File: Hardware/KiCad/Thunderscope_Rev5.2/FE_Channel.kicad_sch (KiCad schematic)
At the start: 103 parts, among them J1002_4 BNC, J3_4 UFL, J4_4 UFL, K1000_4 UD2-4.5NUN-L, K1001_4 UD2-4.5NUN-L, Q1002_4 DMN62D0UW, Q1003_4 DMN62D0UW, U1001_4 TMUX4053, U1008_4 LMH6518, U1009_4 BUF802, U1011_4 OPA140AIDBVR

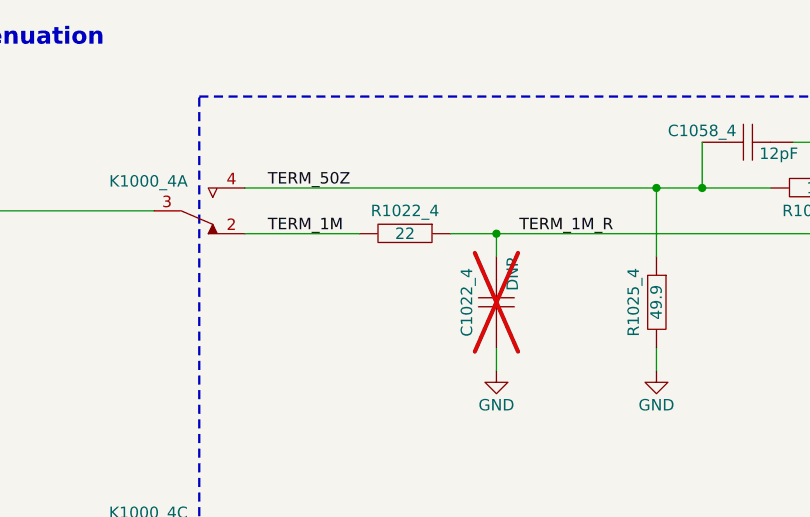
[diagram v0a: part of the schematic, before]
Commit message: Changed R1022 for #387
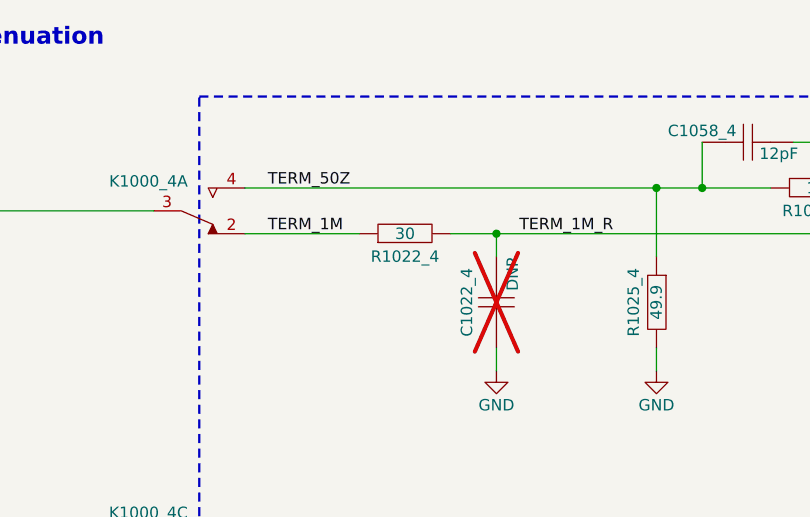
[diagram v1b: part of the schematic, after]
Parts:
- R1022_4: value 22 -> 30; symbol Thunderscope_Rev5:RES 22 OHM 1% 1/3W 0603 -> Thunderscope_Rev5:RES 30 OHM 1% 1/3W 0603; MANUFACTURER PART NUMBER SG73P1JTTD22R0F -> SG73P1JTTD30R0F; SUPPLIER PART NUMBER 1 660-SG73P1JTTD22R0F -> 660-SG73P1JTTD30R0F
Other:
- moved on the sheet: R1022_4
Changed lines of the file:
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@@
 	)
 	(symbol
-		(lib_id "Thunderscope_Rev5:RES 22 OHM 1% 1/3W 0603")
-		(at 91.44 38.1 0)
+		(lib_id "Thunderscope_Rev5:RES 30 OHM 1% 1/3W 0603")
+		(at 91.44 38.1 180)
 		(unit 1)
 		(exclude_from_sim no)
@@
 		(dnp no)
 		(property "Reference" "R1022_4"
-			(at 91.44 35.56 0)
+			(at 91.44 40.64 0)
 			(effects
 				(font
@@
 			)
 		)
-		(property "Value" "22"
+		(property "Value" "30"
 			(at 91.44 38.1 0)
 			(effects
@@
 		)
 		(property "TOLERANCE" "1%"
-			(at 88.392 46.736 0)
+			(at 94.488 29.464 0)
 			(effects
 				(font
@@
 		)
 		(property "PACKAGE" "0603"
-			(at 88.9 40.64 0)
+			(at 93.98 35.56 0)
 			(effects
 				(font
@@
 		)
 		(property "SUPPLIER 1" "Mouser"
-			(at 85.852 34.584 0)
+			(at 97.028 41.616 0)
 			(effects
 				(font
@@
 			)
 		)
-		(property "SUPPLIER PART NUMBER 1" "660-SG73P1JTTD22R0F"
-			(at 85.852 34.584 0)
+		(property "SUPPLIER PART NUMBER 1" "660-SG73P1JTTD30R0F"
+			(at 97.028 41.616 0)
 			(effects
 				(font
@@
 		)
 		(property "MANUFACTURER" "KOA Speer"
-			(at 85.852 34.584 0)
+			(at 97.028 41.616 0)
 			(effects
 				(font
@@
 		)
 		(property "HOUSE PART NUMBER" ""
-			(at 85.852 34.584 0)
+			(at 97.028 41.616 0)
 			(effects
 				(font
@@
 			)
 		)
-		(property "MANUFACTURER PART NUMBER" "SG73P1JTTD22R0F"
-			(at 85.852 34.584 0)
+		(property "MANUFACTURER PART NUMBER" "SG73P1JTTD30R0F"
+			(at 97.028 41.616 0)
 			(effects
 				(font

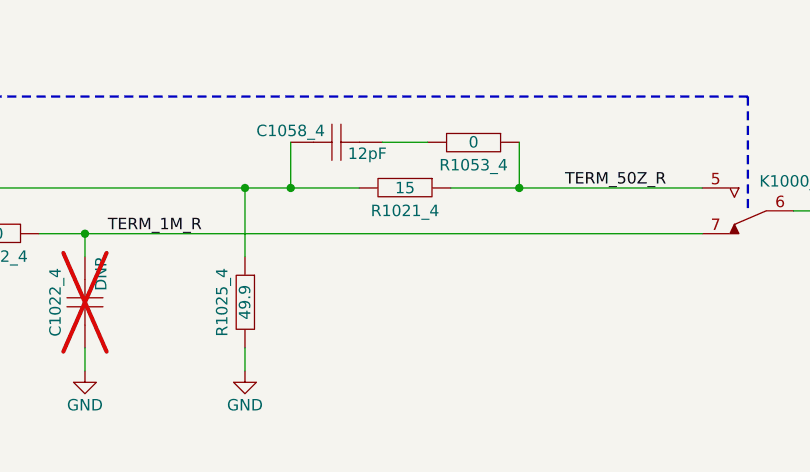
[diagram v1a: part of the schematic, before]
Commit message: Changed R1021 for #388
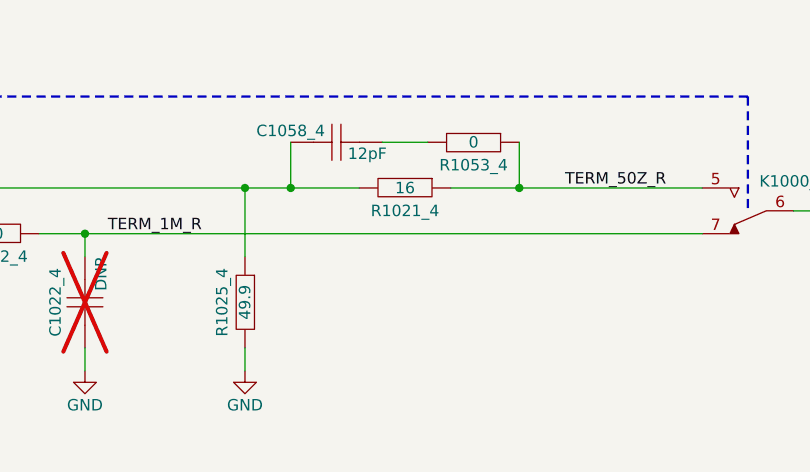
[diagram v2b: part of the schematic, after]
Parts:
- R1021_4: value 15 -> 16; symbol Thunderscope_Rev5:RES 15 OHM 1% 1/3W 0603 -> Thunderscope_Rev5:RES 16 OHM 1% 1/3W 0603; MANUFACTURER PART NUMBER SG73P1JTTD15R0F -> SG73P1JTTD16R0F; SUPPLIER PART NUMBER 1 660-SG73P1JTTD15R0F -> 660-SG73P1JTTD16R0F
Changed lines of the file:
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@@
 	)
 	(symbol
-		(lib_id "Thunderscope_Rev5:RES 15 OHM 1% 1/3W 0603")
+		(lib_id "Thunderscope_Rev5:RES 16 OHM 1% 1/3W 0603")
 		(at 137.16 33.02 0)
 		(unit 1)
@@
 			)
 		)
-		(property "Value" "15"
+		(property "Value" "16"
 			(at 137.16 33.02 0)
 			(effects
@@
 			)
 		)
-		(property "SUPPLIER PART NUMBER 1" "660-SG73P1JTTD15R0F"
+		(property "SUPPLIER PART NUMBER 1" "660-SG73P1JTTD16R0F"
 			(at 131.572 29.504 0)
 			(effects
@@
 			)
 		)
-		(property "MANUFACTURER PART NUMBER" "SG73P1JTTD15R0F"
+		(property "MANUFACTURER PART NUMBER" "SG73P1JTTD16R0F"
 			(at 131.572 29.21 0)
 			(effects

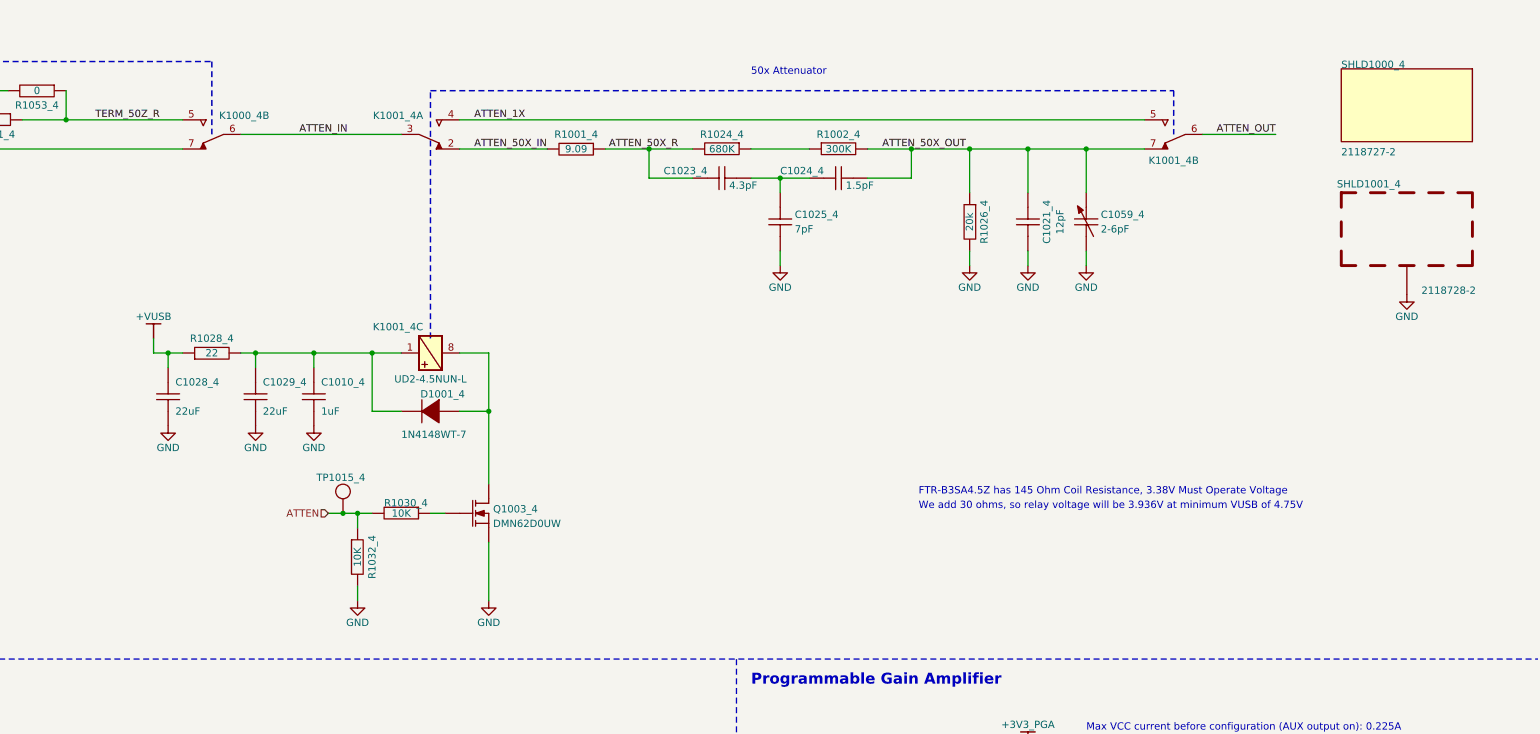
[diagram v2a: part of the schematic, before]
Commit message: Schematic Changes for #389
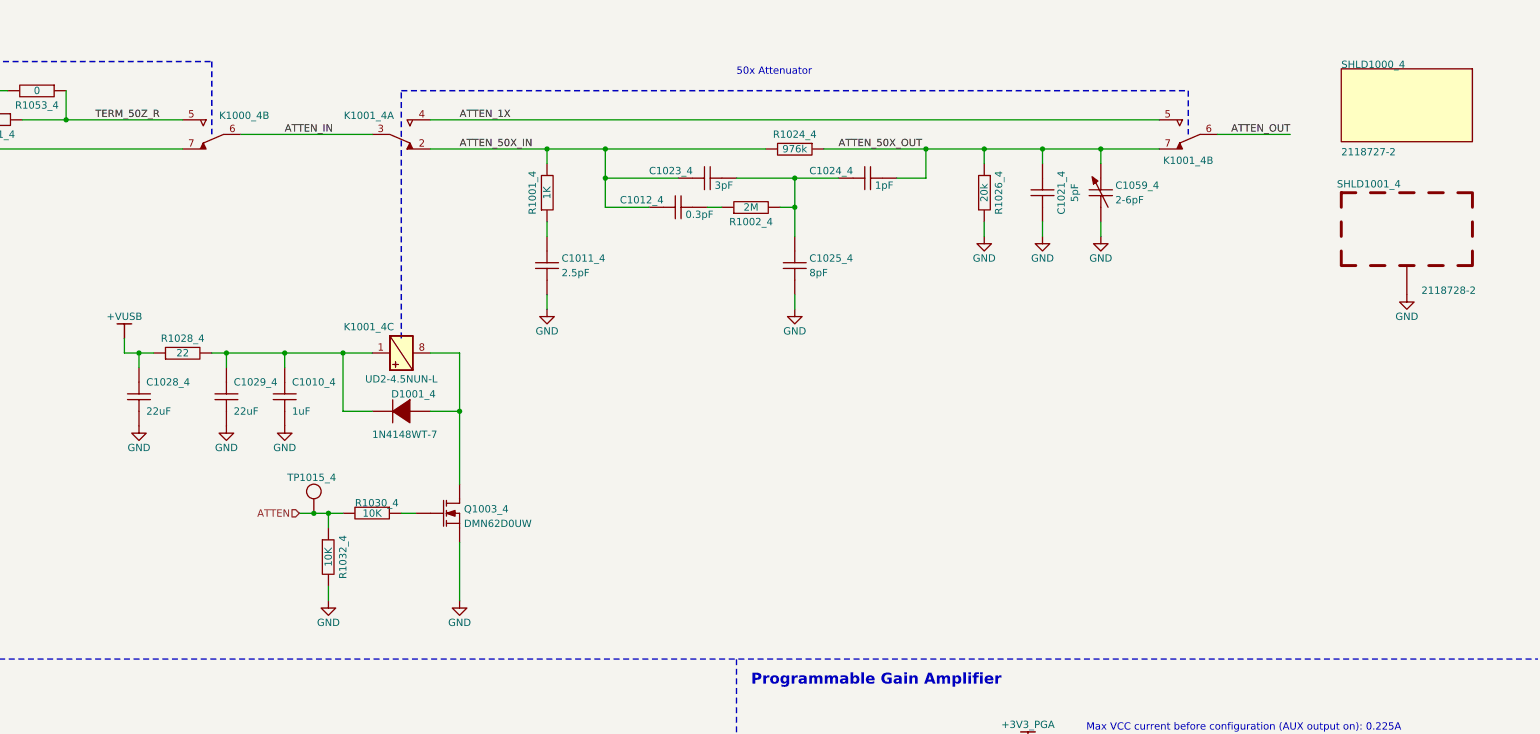
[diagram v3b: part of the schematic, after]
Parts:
- added C1011_4: 2.5pF, Thunderscope_Rev5:GEN_C_0603, symbol Thunderscope_Rev5:CAP 2.5pF 250V C0G 0603
- added C1012_4: 0.3pF, Thunderscope_Rev5:GEN_C_0402, symbol Thunderscope_Rev5:CAP 0.3pF 250V C0G 0402
- C1021_4: value 12pF -> 5pF; symbol Thunderscope_Rev5:CAP 12pF 50V C0G 0402 -> Thunderscope_Rev5:CAP 5pF 50V C0G 0402; MANUFACTURER PART NUMBER CBR04C120F5GAC -> CBR04C509B5GAC; SUPPLIER PART NUMBER 1 80-CBR04C120F5G -> 80-CBR04C509B5G
- C1023_4: value 4.3pF -> 3pF; symbol Thunderscope_Rev5:CAP 4.3pF 250V C0G 0603 -> Thunderscope_Rev5:CAP 3pF 250V C0G 0603; MANUFACTURER PART NUMBER CBR06C439BAGAC -> CBR06C309BAGAC; SUPPLIER PART NUMBER 1 80-CBR06C439BAGAC -> 80-CBR06C309BAG
- C1024_4: value 1.5pF -> 1pF; symbol Thunderscope_Rev5:CAP 1.5pF 50V C0G 0402 -> Thunderscope_Rev5:CAP 1pF 50V C0G 0402; MANUFACTURER PART NUMBER CBR04C159A5GAC -> CBR04C109A5GAC; SUPPLIER PART NUMBER 1 80-CBR04C159A5GAC -> 80-CBR04C109A5GAC
- C1025_4: value 7pF -> 8pF; symbol Thunderscope_Rev5:CAP 7pF 50V C0G 0402 -> Thunderscope_Rev5:CAP 8pF 50V C0G 0402; MANUFACTURER PART NUMBER CBR04C709B5GAC -> CBR04C809B5GAC; SUPPLIER PART NUMBER 1 80-CBR04C709B5GAC -> 80-CBR04C809B5GAC
- R1001_4: value 9.09 -> 1K; symbol Thunderscope_Rev5:RES 9.09 OHM 1% 1/10W 0402 -> Thunderscope_Rev5:RES 1K OHM 1% 1/10W 0402; HOUSE PART NUMBER (none) -> R-1K-0402-1%-001; MANUFACTURER PART NUMBER RC0402FR-079R09L -> RC0402FR-071KL; SUPPLIER PART NUMBER 1 603-RC0402FR-079R09L -> 603-RC0402FR-071KL
- R1002_4: value 300K -> 2M; footprint Thunderscope_Rev5:GEN_R_0402 -> Thunderscope_Rev5:GEN_R_0603; symbol Thunderscope_Rev5:RES 300K OHM 1% 1/10W 0402 -> Thunderscope_Rev5:RES 2M OHM 1% 1/10W 0603; MANUFACTURER Panasonic -> KOA Speer; MANUFACTURER PART NUMBER ERJ-2RKF3003X -> RK73H1JTTD2004F; PACKAGE 0402 -> 0603; SUPPLIER PART NUMBER 1 667-ERJ-2RKF3003X -> 660-RK73H1JTTD2004F
- R1024_4: value 680K -> 976k; footprint Thunderscope_Rev5:GEN_R_0402 -> Thunderscope_Rev5:GEN_R_0603; symbol Thunderscope_Rev5:RES 680K OHM 1% 1/16W 0402 -> Thunderscope_Rev5:RES 976k OHM 1% 1/10W 0603; MANUFACTURER Yageo -> KOA Speer; MANUFACTURER PART NUMBER RC0402FR-07681KL -> RK73H1JTTD9763F; PACKAGE 0402 -> 0603; SUPPLIER PART NUMBER 1 603-RC0402FR-07680KL -> 660-RK73H1JTTD9763F
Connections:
- net ATTEN_50X_IN: now also C1023_4.2, R1001_4.2, R1024_4.1, C1012_4.2; no longer R1001_4.1
- net ATTEN_50X_OUT: now also R1024_4.2; no longer R1002_4.1
- net GND: now also C1011_4.1
- net at R1002_4.2: now also C1023_4.1, C1024_4.2, C1025_4.2; no longer R1024_4.1
- removed net ATTEN_50X_R: C1023_4.2, R1001_4.2, R1024_4.2
- new net: C1012_4.1, R1002_4.1
- new net: C1011_4.2, R1001_4.1
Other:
- note removed: "FTR-B3SA4.5Z has 145 Ohm Coil Resistance, 3.38V Must Operate Voltage"
- note removed: "We add 30 ohms, so relay voltage will be 3.936V at minimum VUSB of 4.75V"
- moved on the sheet: C1010_4, C1021_4, C1023_4, C1024_4, C1025_4, C1028_4, C1029_4, C1059_4, D1001_4, K1001_4A, K1001_4B, K1001_4C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

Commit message: Routed Attenuator for #389 and cutouts for #385
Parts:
- C1011_4: footprint Thunderscope_Rev5:GEN_C_0603 -> Thunderscope_Rev5:GEN_C_0402; symbol Thunderscope_Rev5:CAP 2.5pF 250V C0G 0603 -> Thunderscope_Rev5:CAP 2.5pF 200V C0G 0402; MANUFACTURER PART NUMBER CBR06C259BAGAC -> CBR04C259B2GAC; PACKAGE 0603 -> 0402; SUPPLIER PART NUMBER 1 80-CBR06C259BAGAC -> 80-CBR04C259B2GAC; VOLTAGE RATING 250V -> 200V
- C1023_4: footprint Thunderscope_Rev5:GEN_C_0603 -> Thunderscope_Rev5:GEN_C_0402; symbol Thunderscope_Rev5:CAP 3pF 250V C0G 0603 -> Thunderscope_Rev5:CAP 3pF 200V C0G 0402; MANUFACTURER PART NUMBER CBR06C309BAGAC -> CBR04C309B2GAC; PACKAGE 0603 -> 0402; SUPPLIER PART NUMBER 1 80-CBR06C309BAG -> 80-CBR04C309B2GAC; VOLTAGE RATING 250V -> 200V
- R1002_4: footprint Thunderscope_Rev5:GEN_R_0603 -> Thunderscope_Rev5:GEN_R_0402; symbol Thunderscope_Rev5:RES 2M OHM 1% 1/10W 0603 -> Thunderscope_Rev5:RES 2M OHM 1% 1/10W 0402; MANUFACTURER PART NUMBER RK73H1JTTD2004F -> RK73H1ETTP2004F; PACKAGE 0603 -> 0402; SUPPLIER PART NUMBER 1 660-RK73H1JTTD2004F -> 660-RK73H1ETTP2004F
- R1024_4: footprint Thunderscope_Rev5:GEN_R_0603 -> Thunderscope_Rev5:GEN_R_0402; symbol Thunderscope_Rev5:RES 976k OHM 1% 1/10W 0603 -> Thunderscope_Rev5:RES 976k OHM 1% 1/10W 0402; MANUFACTURER PART NUMBER RK73H1JTTD9763F -> RK73H1ETTP9763F; PACKAGE 0603 -> 0402; SUPPLIER PART NUMBER 1 660-RK73H1JTTD9763F -> 660-RK73H1ETTP9763F
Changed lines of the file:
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@@
 	)
 	(symbol
-		(lib_id "Thunderscope_Rev5:RES 2M OHM 1% 1/10W 0603")
+		(lib_id "Thunderscope_Rev5:RES 2M OHM 1% 1/10W 0402")
 		(at 269.24 48.26 180)
 		(unit 1)
@@
 			)
 		)
-		(property "Footprint" "Thunderscope_Rev5:GEN_R_0603"
+		(property "Footprint" "Thunderscope_Rev5:GEN_R_0402"
 			(at 269.24 48.26 0)
 			(effects
@@
 			)
 		)
-		(property "PACKAGE" "0603"
+		(property "PACKAGE" "0402"
 			(at 269.24 48.26 0)
 			(effects
@@
 			)
 		)
-		(property "SUPPLIER PART NUMBER 1" "660-RK73H1JTTD2004F"
+		(property "SUPPLIER PART NUMBER 1" "660-RK73H1ETTP2004F"
 			(at 269.24 48.26 0)
 			(effects
@@
 			)
 		)
-		(property "MANUFACTURER PART NUMBER" "RK73H1JTTD2004F"
+		(property "MANUFACTURER PART NUMBER" "RK73H1ETTP2004F"
 			(at 269.24 48.26 0)
 			(effects
@@
 	)
 	(symbol
-		(lib_id "Thunderscope_Rev5:RES 976k OHM 1% 1/10W 0603")
+		(lib_id "Thunderscope_Rev5:RES 976k OHM 1% 1/10W 0402")
 		(at 276.86 38.1 0)
 		(unit 1)
@@
 			)
 		)
-		(property "Footprint" "Thunderscope_Rev5:GEN_R_0603"
+		(property "Footprint" "Thunderscope_Rev5:GEN_R_0402"
 			(at 276.86 38.1 0)
 			(effects
@@
 			)
 		)
-		(property "PACKAGE" "0603"
+		(property "PACKAGE" "0402"
 			(at 273.812 46.736 0)
 			(effects
@@
 			)
 		)
-		(property "MANUFACTURER PART NUMBER" "RK73H1JTTD9763F"
+		(property "MANUFACTURER PART NUMBER" "RK73H1ETTP9763F"
 			(at 271.272 34.584 0)
 			(effects
@@
 			)
 		)
-		(property "SUPPLIER PART NUMBER 1" "660-RK73H1JTTD9763F"
+		(property "SUPPLIER PART NUMBER 1" "660-RK73H1ETTP9763F"
 			(at 271.272 34.584 0)
 			(effects
@@
 	)
 	(symbol
-		(lib_id "Thunderscope_Rev5:CAP 3pF 250V C0G 0603")
+		(lib_id "Thunderscope_Rev5:CAP 3pF 200V C0G 0402")
 		(at 261.62 43.18 0)
 		(unit 1)
@@
 			)
 		)
-		(property "Footprint" "Thunderscope_Rev5:GEN_C_0603"
+		(property "Footprint" "Thunderscope_Rev5:GEN_C_0402"
 			(at 261.62 43.18 0)
 			(effects
@@
 			)
 		)
-		(property "PACKAGE" "0603"
+		(property "PACKAGE" "0402"
 			(at 259.08 52.07 0)
 			(effects
@@
 			)
 		)
-		(property "SUPPLIER PART NUMBER 1" "80-CBR06C309BAG"
+		(property "SUPPLIER PART NUMBER 1" "80-CBR04C309B2GAC"
 			(at 256.032 40.926 0)
 			(effects
@@
 			)
 		)
-		(property "VOLTAGE RATING" "250V"
+		(property "VOLTAGE RATING" "200V"
 			(at 259.08 54.61 0)
 			(effects
@@
 			)
 		)
-		(property "MANUFACTURER PART NUMBER" "CBR06C309BAGAC"
+		(property "MANUFACTURER PART NUMBER" "CBR04C309B2GAC"
 			(at 259.366 37.592 0)
 			(effects
@@
 	)
 	(symbol
-		(lib_id "Thunderscope_Rev5:CAP 2.5pF 250V C0G 0603")
+		(lib_id "Thunderscope_Rev5:CAP 2.5pF 200V C0G 0402")
 		(at 233.68 58.42 270)
 		(unit 1)
@@
 			)
 		)
-		(property "Footprint" "Thunderscope_Rev5:GEN_C_0603"
+		(property "Footprint" "Thunderscope_Rev5:GEN_C_0402"
 			(at 233.68 58.42 0)
 			(effects
@@
 			)
 		)
-		(property "PACKAGE" "0603"
+		(property "PACKAGE" "0402"
 			(at 224.79 55.88 0)
 			(effects
@@
 			)
 		)
-		(property "SUPPLIER PART NUMBER 1" "80-CBR06C259BAGAC"
+		(property "SUPPLIER PART NUMBER 1" "80-CBR04C259B2GAC"
 			(at 235.934 52.832 0)
 			(effects
@@
 			)
 		)
-		(property "VOLTAGE RATING" "250V"
+		(property "VOLTAGE RATING" "200V"
 			(at 222.25 55.88 0)
 			(effects
@@
 			)
 		)
-		(property "MANUFACTURER PART NUMBER" "CBR06C259BAGAC"
+		(property "MANUFACTURER PART NUMBER" "CBR04C259B2GAC"
 			(at 239.268 56.166 0)
 			(effects
